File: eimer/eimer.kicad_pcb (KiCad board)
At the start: 2 copper layers, 77.8 x 67.9 mm, 71 parts, among them J3 Conn_01x03, J4 USB_C_Receptacle_USB2.0_14P, SW1 SW_Push, SW2 SW_Push, U1 RP2040, U2 MCP1700x-330xxTT, U3 TPS61221DCK, U4 W25Q16JVUXIQ TR, U5 LIS2DW12, Y1 12 MHz

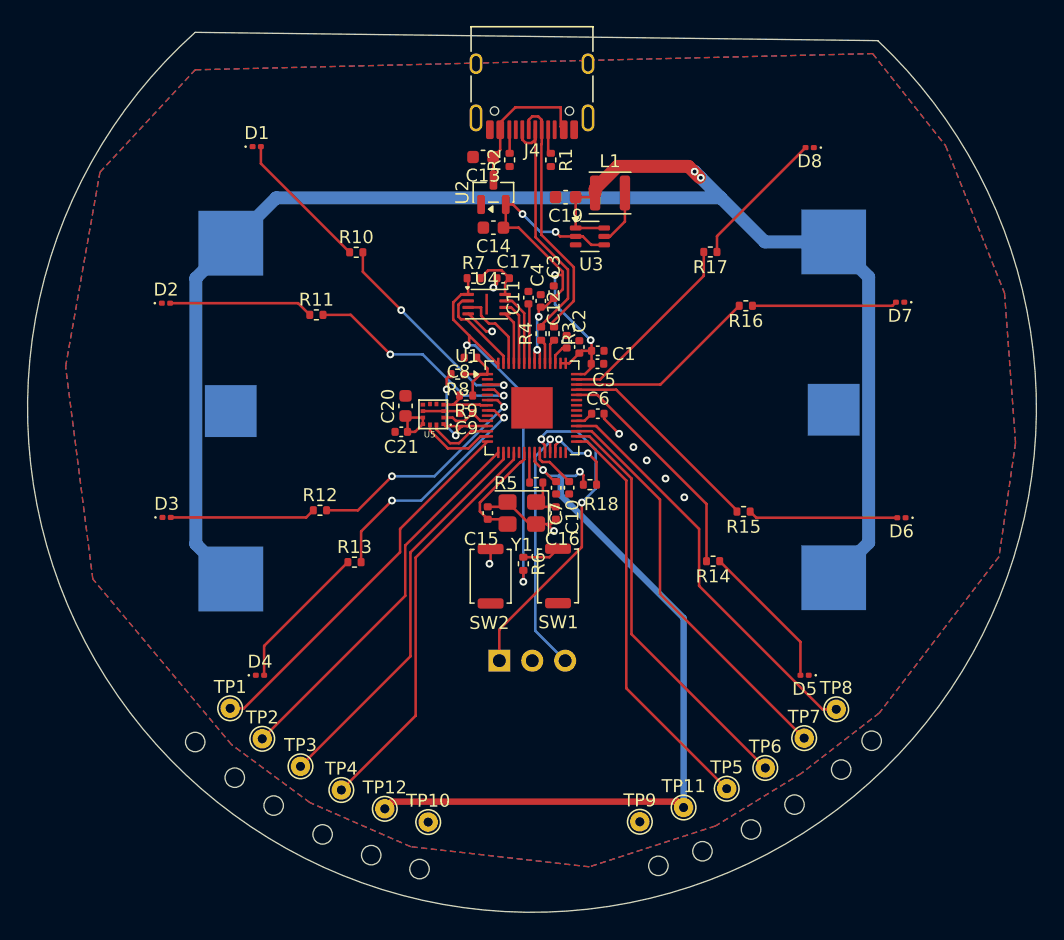
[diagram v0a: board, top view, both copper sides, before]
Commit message: finished all routing
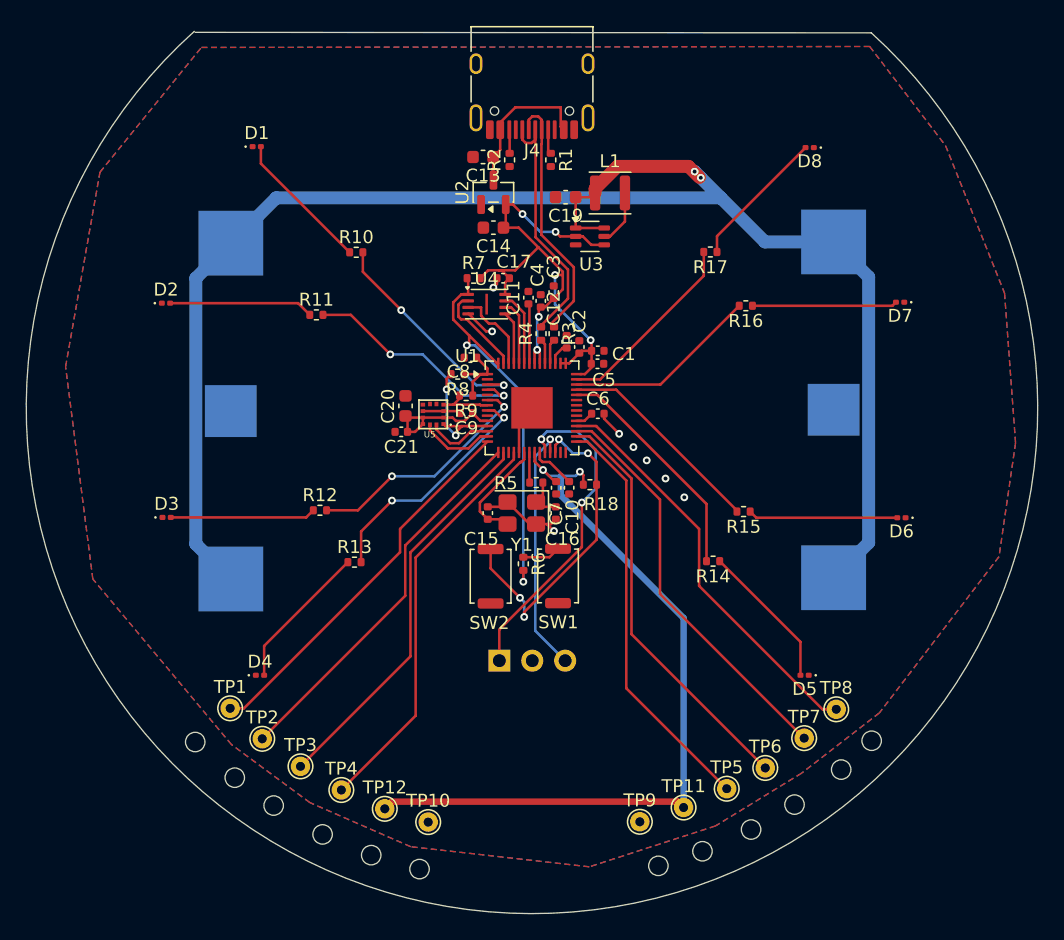
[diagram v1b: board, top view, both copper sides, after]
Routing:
- net Net-(U1-RUN): track 7.69 -> 25.3 mm, vias 3 -> 4
- net +3.3V: track 119.0 -> 124.3 mm
- net GND: track 15.2 -> 19.1 mm
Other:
- board size 77.8 x 67.9 mm -> 78 x 68.1 mm
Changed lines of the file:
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@@
 		(layer "Edge.Cuts")
 	)
-	(gr_circle
-		(center 100.025 114.7)
-		(end 100.775 114.7)
+	(gr_arc
+		(start 100 60.1)
+		(mid 73.738464 128.034983)
+		(end 47.778586 59.984157)
 		(stroke
 			(width 0.05)
-			(type solid)
+			(type default)
 		)
-		(fill no)
 		(layer "Edge.Cuts")
 	)
 	(gr_line
-		(start 100.5 60.700002)
+		(start 100 60.1)
 		(end 47.8465 60.059871)
 		(stroke
@@
 		(layer "Edge.Cuts")
 	)
-	(gr_arc
-		(start 100.5 60.7)
-		(mid 73.352011 127.930495)
-		(end 47.846498 60.059871)
+	(gr_circle
+		(center 100.025 114.7)
+		(end 100.775 114.7)
 		(stroke
 			(width 0.05)
-			(type default)
+			(type solid)
 		)
+		(fill no)
 		(layer "Edge.Cuts")
 	)
@@
 	)
 	(segment
+		(start 72.826461 90.024888)
+		(end 73.826461 89.024888)
+		(width 0.2)
+		(layer "F.Cu")
+		(net "GND")
+	)
+	(segment
 		(start 74.14 97.9875)
 		(end 73.64 97.9875)
@@
 	)
 	(segment
+		(start 72.826461 92.462388)
+		(end 72.826461 90.024888)
+		(width 0.2)
+		(layer "F.Cu")
+		(net "GND")
+	)
+	(segment
 		(start 75.525 98.525)
 		(end 75.025 98.025)
@@
 	)
 	(segment
-		(start 76.201461 78.526359)
+		(start 74.312551 76.637449)
 		(end 72.79999 75.124888)
 		(width 0.2)
@@
 	)
 	(segment
+		(start 65.4075 89.775)
+		(end 67.0075 89.775)
+		(width 0.2)
+		(layer "F.Cu")
+		(net "+3.3V")
+	)
+	(segment
 		(start 76.426461 85.587388)
 		(end 76.693961 85.587388)
@@
 	)
 	(segment
+		(start 71.3 78.414888)
+		(end 72.535112 78.414888)
+		(width 0.2)
+		(layer "F.Cu")
+		(net "+3.3V")
+	)
+	(segment
 		(start 78.396461 85.624888)
 		(end 78.396461 85.934887)
@@
 	)
 	(segment
+		(start 70.446461 78.414888)
+		(end 71.3 78.414888)
+		(width 0.2)
+		(layer "F.Cu")
+		(net "+3.3V")
+	)
+	(segment
 		(start 74.426461 84.749888)
 		(end 74.226461 84.549888)
@@
 	)
 	(segment
+		(start 76.201461 78.526359)
+		(end 74.312551 76.637449)
+		(width 0.2)
+		(layer "F.Cu")
+		(net "+3.3V")
+	)
+	(segment
 		(start 77.195 75.8)
 		(end 75.995 75.8)
@@
 	)
 	(segment
+		(start 72.535112 78.414888)
+		(end 74.312551 76.637449)
+		(width 0.2)
+		(layer "F.Cu")
+		(net "+3.3V")
+	)
+	(segment
 		(start 74.026461 84.749888)
 		(end 74.226461 84.549888)
@@
 	)
 	(segment
-		(start 70.446461 78.414888)
+		(start 71.3 78.414888)
 		(end 71.471461 78.414888)
 		(width 0.2)
@@
 	)
 	(segment
-		(start 70.633539 100.961461)
-		(end 70.545 101.05)
+		(start 78.805 94.95)
+		(end 78.805 99.194485)
 		(width 0.2)
 		(layer "F.Cu")
@@
 	)
 	(segment
+		(start 75.626461 91.898417)
+		(end 75.901461 91.623417)
+		(width 0.2)
+		(layer "F.Cu")
+		(net "Net-(U1-RUN)")
+	)
+	(segment
+		(start 70.633539 101.408539)
+		(end 72.9 103.675)
+		(width 0.2)
+		(layer "F.Cu")
+		(net "Net-(U1-RUN)")
+	)
+	(segment
 		(start 70.633539 99.912612)
-		(end 70.633539 100.961461)
+		(end 70.633539 101.408539)
 		(width 0.2)
 		(layer "F.Cu")
@@
 	)
 	(segment
-		(start 75.626461 91.898417)
-		(end 75.901461 91.623417)
+		(start 73.225 104.774485)
+		(end 73.225 105.15)
 		(width 0.2)
 		(layer "F.Cu")
@@
 		(net "Net-(U1-RUN)")
 	)
+	(segment
+		(start 78.805 99.194485)
+		(end 73.225 104.774485)
+		(width 0.2)
+		(layer "F.Cu")
+		(net "Net-(U1-RUN)")
+	)
 	(via
 		(at 75.901461 91.449888)
@@
 	)
 	(via
-		(at 70.545 101.05)
+		(at 72.9 103.675)
 		(size 0.6)
 		(drill 0.3)
 		(layers "F.Cu" "B.Cu")
-		(free yes)
 		(net "Net-(U1-RUN)")
 	)
@@
 		(net "Net-(U1-RUN)")
 	)
+	(via
+		(at 73.225 105.15)
+		(size 0.6)
+		(drill 0.3)
+		(layers "F.Cu" "B.Cu")
+		(net "Net-(U1-RUN)")
+	)
+	(segment
+		(start 73.225 104)
+		(end 72.9 103.675)
+		(width 0.2)
+		(layer "B.Cu")
+		(net "Net-(U1-RUN)")
+	)
+	(segment
+		(start 73.225 105.15)
+		(end 73.225 104)
+		(width 0.2)
+		(layer "B.Cu")
+		(net "Net-(U1-RUN)")
+	)
 	(segment
 		(start 76.976573 92.525)
@@
 		(polygon
 			(pts
-				(xy 100.1 61.7) (xy 105.725 68.8) (xy 110.275 80.175) (xy 111.125 91.725) (xy 109.85 100.5) (xy 100.625 112.55)
+				(xy 99.875 61.15) (xy 105.725 68.8) (xy 110.275 80.175) (xy 111.125 91.725) (xy 109.85 100.5) (xy 100.625 112.55)
 				(xy 94.625 117.2) (xy 87.975 121.275) (xy 78.25 124.425) (xy 64.475 122.875) (xy 56.7 119.475) (xy 50.65 115)
-				(xy 39.95 102.225) (xy 37.85 85.85) (xy 40.5 70.85) (xy 47.85 62.95)
+				(xy 39.95 102.225) (xy 37.85 85.85) (xy 40.5 70.85) (xy 48.325 61.225)
 			)
 		)
